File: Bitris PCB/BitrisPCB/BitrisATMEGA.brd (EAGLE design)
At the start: 49.2 x 50.8 mm, 27 parts, among them IC1 ATMEGA328-20P, IC2 4511N, X1 Boton, X2 Sonido, X3 Alimentacion, X4 22-23-2021

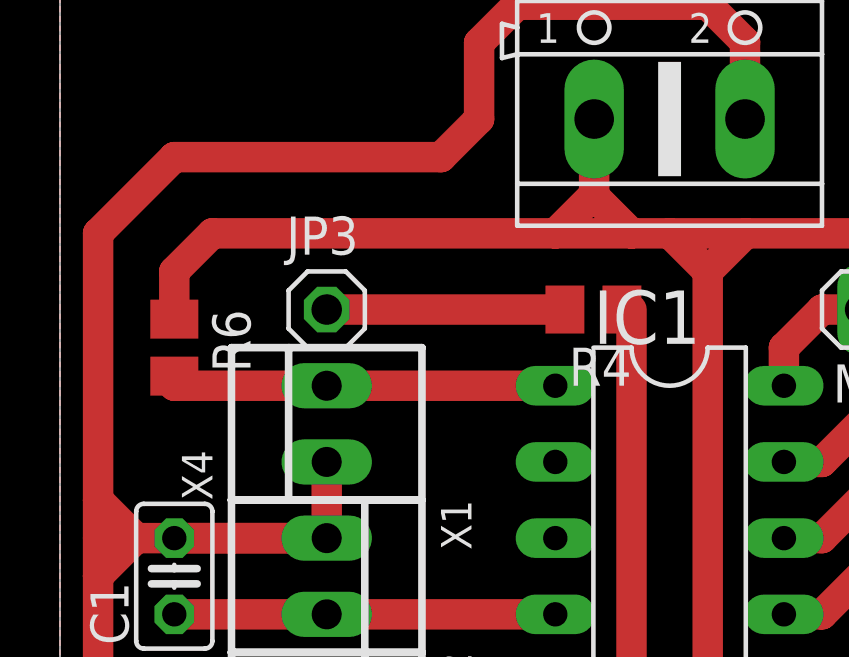
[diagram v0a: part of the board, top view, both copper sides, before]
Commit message: PCB modificado
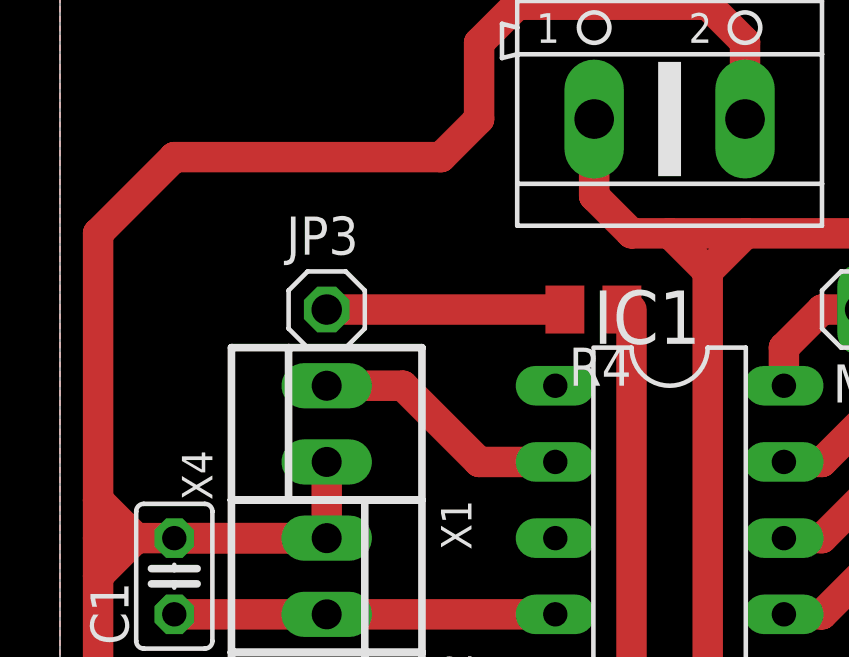
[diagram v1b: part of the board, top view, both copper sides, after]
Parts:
- removed R6: (no value), rcl:M0805
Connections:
- removed net N$34: IC1.1, R6.2, X4.2
- new net N$30: IC1.2, X4.2
- net VCC: no longer R6.1
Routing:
- net VCC: track 122.5 -> 103.3 mm
- net N$34: track 13.0 -> 0.00 mm
- net N$30: track 0.00 -> 8.67 mm
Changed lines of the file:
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@@
 <attribute name="SPICEPREFIX" value="R" x="78.74" y="38.1" size="1.778" layer="27" display="off"/>
-</element>
-<element name="R6" library="rcl" package="M0805" value="" x="39.37" y="46.99" rot="R270">
-<attribute name="SPICEPREFIX" value="R" x="39.37" y="46.99" size="1.778" layer="27" rot="R270" display="off"/>
 </element>
 <element name="R7" library="rcl" package="M0805" value="" x="78.74" y="40.64">
@@
 <contactref element="X3" pad="1"/>
 <contactref element="IC2" pad="16"/>
-<contactref element="R6" pad="1"/>
 <wire x1="67.31" y1="38.1" x2="67.31" y2="39.37" width="1.016" layer="1"/>
 <wire x1="52.07" y1="30.48" x2="54.61" y2="30.48" width="1.016" layer="1"/>
@@
 <wire x1="54.61" y1="50.8" x2="55.88" y2="50.8" width="1.016" layer="1"/>
 <wire x1="55.88" y1="50.8" x2="57.15" y2="49.53" width="1.016" layer="1"/>
-<wire x1="39.37" y1="47.94" x2="39.37" y2="49.53" width="1.016" layer="1"/>
-<wire x1="39.37" y1="49.53" x2="40.64" y2="50.8" width="1.016" layer="1"/>
-<wire x1="40.64" y1="50.8" x2="52.07" y2="50.8" width="1.016" layer="1"/>
-<wire x1="52.07" y1="50.8" x2="54.61" y2="50.8" width="1.016" layer="1"/>
 <wire x1="59.69" y1="27.94" x2="59.69" y2="25.4" width="1.016" layer="1"/>
 <wire x1="55.88" y1="50.8" x2="58.42" y2="50.8" width="1.016" layer="1"/>
@@
 <wire x1="74.93" y1="45.72" x2="73.66" y2="45.72" width="1.016" layer="1"/>
 <wire x1="73.66" y1="45.72" x2="72.39" y2="45.72" width="1.016" layer="1"/>
-<wire x1="52.07" y1="50.8" x2="53.34" y2="52.07" width="1.016" layer="1"/>
 <wire x1="72.39" y1="44.45" x2="73.66" y2="45.72" width="1.016" layer="1"/>
 <wire x1="73.66" y1="45.72" x2="72.39" y2="46.99" width="1.016" layer="1"/>
@@
 <wire x1="39.37" y1="38.1" x2="44.45" y2="38.1" width="1.016" layer="1"/>
 </signal>
-<signal name="N$34">
-<contactref element="IC1" pad="1"/>
-<contactref element="R6" pad="2"/>
-<contactref element="X4" pad="2"/>
-<wire x1="52.07" y1="45.72" x2="44.45" y2="45.72" width="1.016" layer="1"/>
-<wire x1="44.45" y1="45.72" x2="39.37" y2="45.72" width="1.016" layer="1"/>
-<wire x1="39.37" y1="45.72" x2="39.37" y2="46.04" width="1.016" layer="1"/>
-</signal>
 <signal name="N$23">
 <contactref element="IC2" pad="10"/>
@@
 <wire x1="48.26" y1="17.78" x2="52.07" y2="17.78" width="1.016" layer="1"/>
 </signal>
+<signal name="N$30">
+<contactref element="IC1" pad="2"/>
+<contactref element="X4" pad="2"/>
+<wire x1="52.07" y1="43.18" x2="49.53" y2="43.18" width="1.016" layer="1"/>
+<wire x1="49.53" y1="43.18" x2="46.99" y2="45.72" width="1.016" layer="1"/>
+<wire x1="46.99" y1="45.72" x2="44.45" y2="45.72" width="1.016" layer="1"/>
+</signal>
 </signals>
